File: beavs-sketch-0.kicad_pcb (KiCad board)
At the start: 4 copper layers, 51.9 x 165.1 mm, 52 parts, among them J1 USB_C_Receptacle_USB2.0_16P, J10 Conn_01x03, J11 Conn_01x03, J12 Micro_SD_Card, J2 Conn_Coaxial, J3 Conn_01x02, J4 Conn_Coaxial, J5 Conn_01x02, J6 Conn_01x03, J7 Conn_01x03, J8 Conn_01x03, J9 Conn_01x03, Q2 SiS427EDN, U1 RP2040, U10 INA745A, U11 INA745A, U12 INA745A, U13 INA745A, U14 ISM6HG256X, U15 SN74LVC8T245, U2 W25Q128JVS, U3 MS5607-02BA, U4 RFM95W-915S2, U5 MAX-M10S, U6 INA745A, U7 AMS1117-3.3, U8 AMS1117-5.0, U9 INA745A, Y1 Crystal_GND24

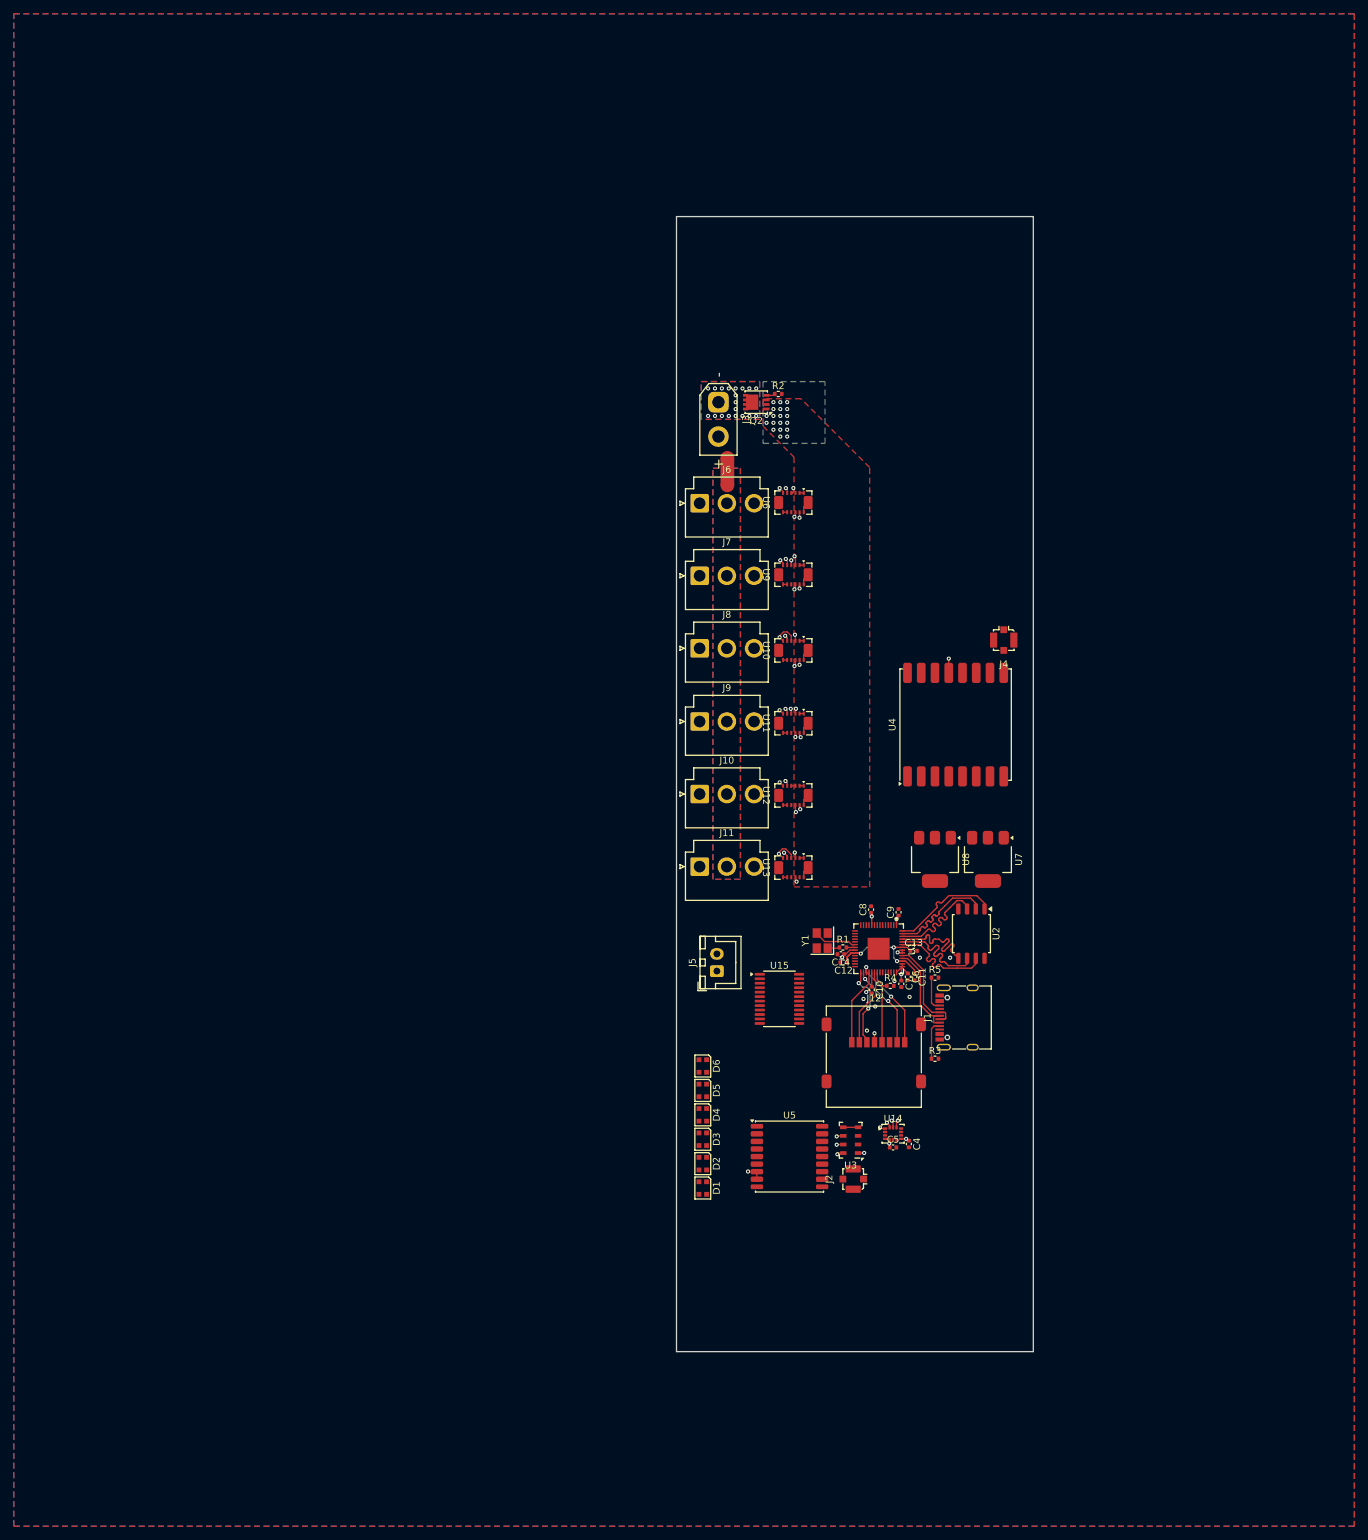
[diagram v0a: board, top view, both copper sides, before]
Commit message: got it to fit in about the right shape
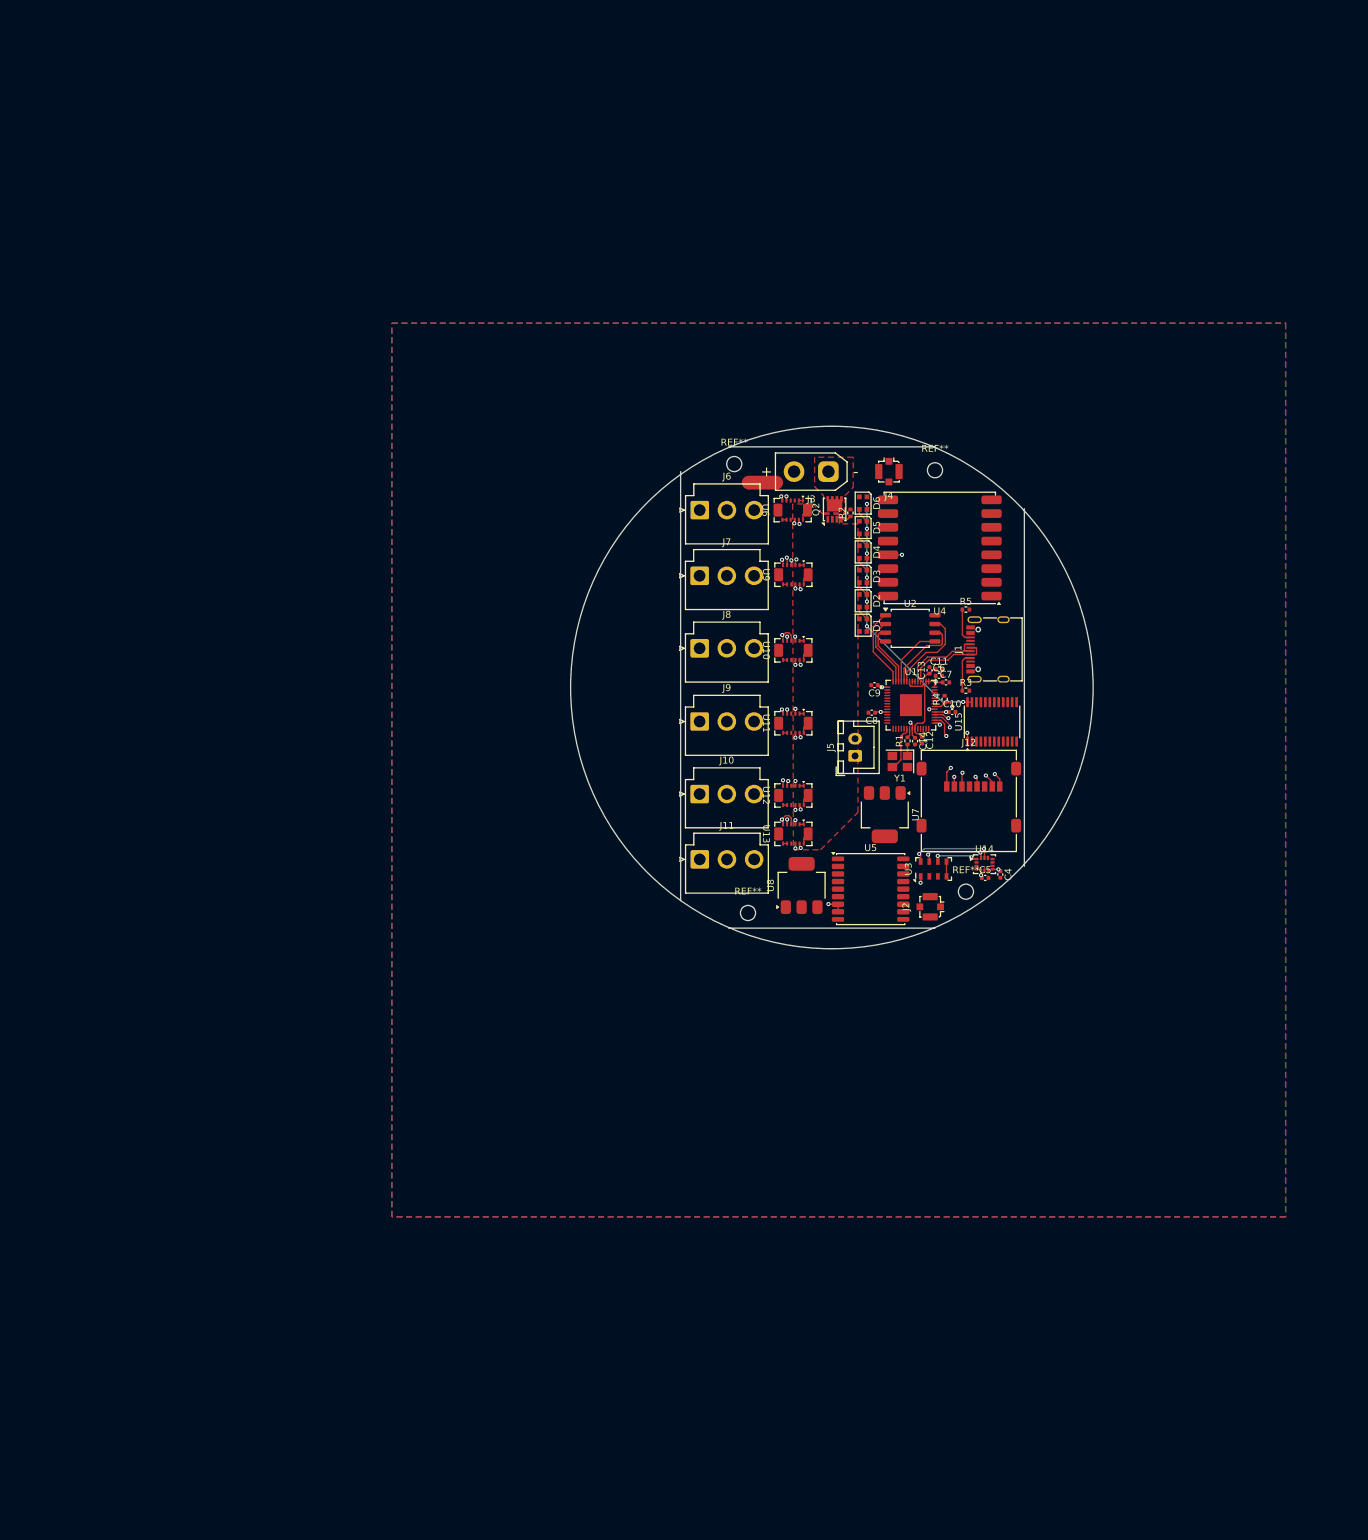
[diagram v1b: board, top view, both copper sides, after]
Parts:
- added REF**: MountingHole_2.2mm_M2, MountingHole:MountingHole_2.2mm_M2, F.Cu at (214.0, 56.4)
- added REF**: MountingHole_2.2mm_M2, MountingHole:MountingHole_2.2mm_M2, F.Cu at (186.8, 120.8)
- added REF**: MountingHole_2.2mm_M2, MountingHole:MountingHole_2.2mm_M2, F.Cu at (184.8, 55.5)
- added REF**: MountingHole_2.2mm_M2, MountingHole:MountingHole_2.2mm_M2, F.Cu at (218.5, 117.7)
- moved D3 85.1 mm to (203.6, 71.8)
- moved D1 85.1 mm to (203.6, 78.9)
- moved D4 85.1 mm to (203.6, 68.3)
- moved D6 85.1 mm to (203.6, 61.2)
- moved D2 85.1 mm to (203.6, 75.4)
- moved D5 85.1 mm to (203.6, 64.7)
- moved J1 53.7 mm to (222.9, 82.5)
- moved R3 53.7 mm to (218.5, 88.5)
- moved R5 53.7 mm to (218.5, 76.7)
- moved U15 50.8 mm to (222.3, 93.0), turned to 90 degrees
- moved U2 45.3 mm to (210.4, 79.4), turned to 0 degrees
- moved C11 44.9 mm to (214.6, 85.4), turned to 0 degrees
- moved C7 44.3 mm to (215.6, 87.3), turned to 0 degrees
- moved C6 44.0 mm to (214.6, 86.3), turned to 0 degrees
- moved R4 42.4 mm to (215.4, 89.7), turned to 90 degrees
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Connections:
- U15 pad 1: unconnected-(U15-V_{CCA}-Pad1) -> +3V3
- U15 pad 11: Net-(U15-GND-Pad11) -> GND
- U15 pad 12: Net-(U15-GND-Pad11) -> GND
- U15 pad 13: Net-(U15-GND-Pad11) -> GND
- U15 pad 23: Net-(U15-V_{CCB}-Pad23) -> +5V
- U15 pad 24: Net-(U15-V_{CCB}-Pad23) -> +5V
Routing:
- net +5V: track 0.00 -> 42.2 mm, vias 0 -> 7
- net /servos/SCL: track 64.2 -> 57.0 mm
- net /servos/SDA: track 58.3 -> 51.5 mm
- net Net-(U1-QSPI_SD0): track 15.9 -> 9.13 mm
- net Net-(U1-QSPI_SD2): track 16.0 -> 9.24 mm
- net /SD Card/CLK: track 11.2 -> 17.6 mm, vias 0 -> 2
- net Net-(U1-QSPI_SD1): track 15.9 -> 10.3 mm
- net +1V1: track 19.7 -> 15.3 mm, vias 3 -> 0
- net Net-(U1-QSPI_SCLK): track 15.9 -> 11.5 mm
- net Net-(U1-QSPI_SS): track 16.0 -> 11.7 mm
- net /SD Card/DAT2: track 11.2 -> 14.7 mm, vias 0 -> 2
- net Net-(U1-QSPI_SD3): track 15.9 -> 12.7 mm
- net /Sensors/MISO: track 9.29 -> 6.66 mm
- net /SD Card/DAT3: track 11.2 -> 13.5 mm, vias 0 -> 2
- net +3V3: track 31.5 -> 29.3 mm
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- removed copper zone on B.Cu, net +BATT
- removed copper zone on B.Cu, net GND1
- removed copper zone on F.Cu, net GND1
- removed copper zone on B.Cu, net Net-(J3-Pin_1)
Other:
- board size 51.9 x 165.1 mm -> 76 x 76 mm
